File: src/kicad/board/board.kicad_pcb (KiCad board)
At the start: 2 copper layers, 109.4 x 83.4 mm, 50 parts, among them J1 Screw_Terminal_Speaker, J2 Micro_SD_Card_Det, Q1 DMG2301L, SW1 SW_Keyboard, SW2 SW_Keyboard, SW3 RotEncoder_S, SW4 SW_Keyboard, SW5 SW_Keyboard, SW6 Enable BAT, U1 Pico, U2 MAX98357, U3 BQ25172, U5 74HC4051, U6 4072

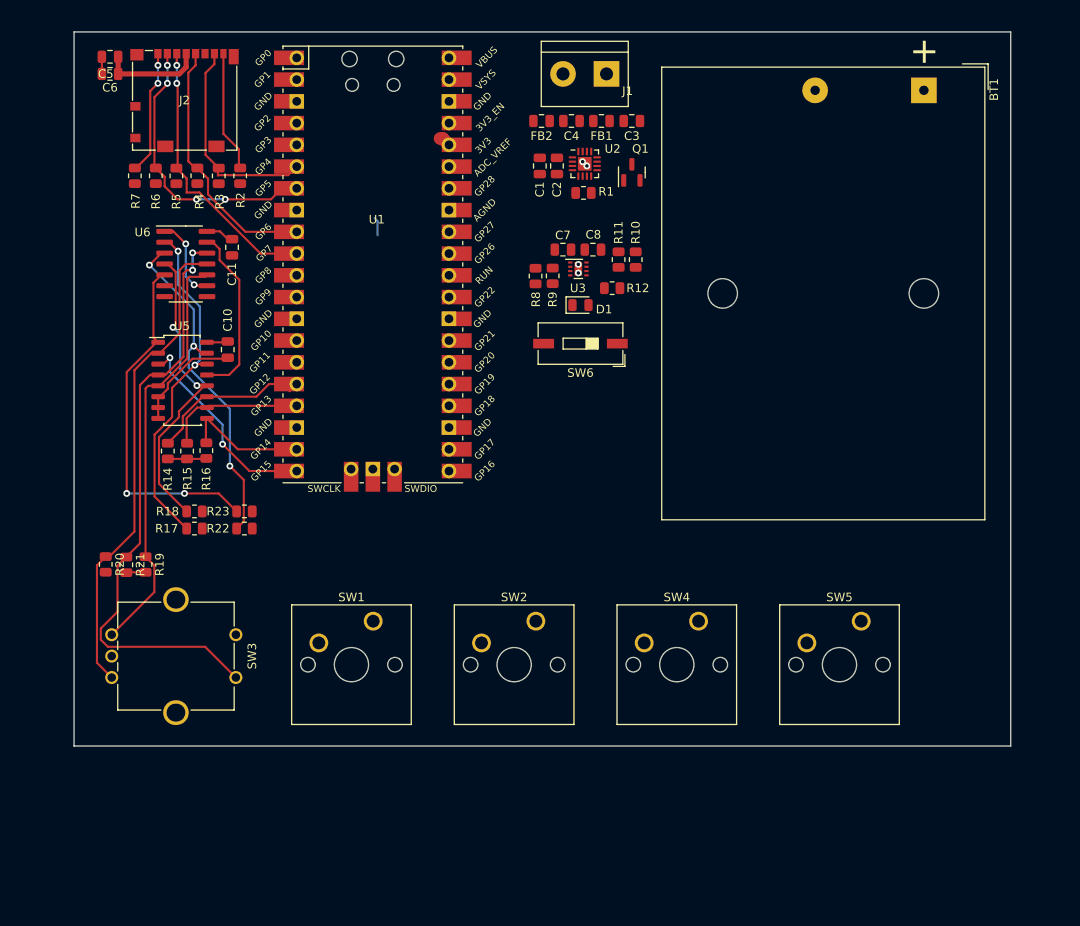
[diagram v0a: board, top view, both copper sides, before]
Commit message: update wip
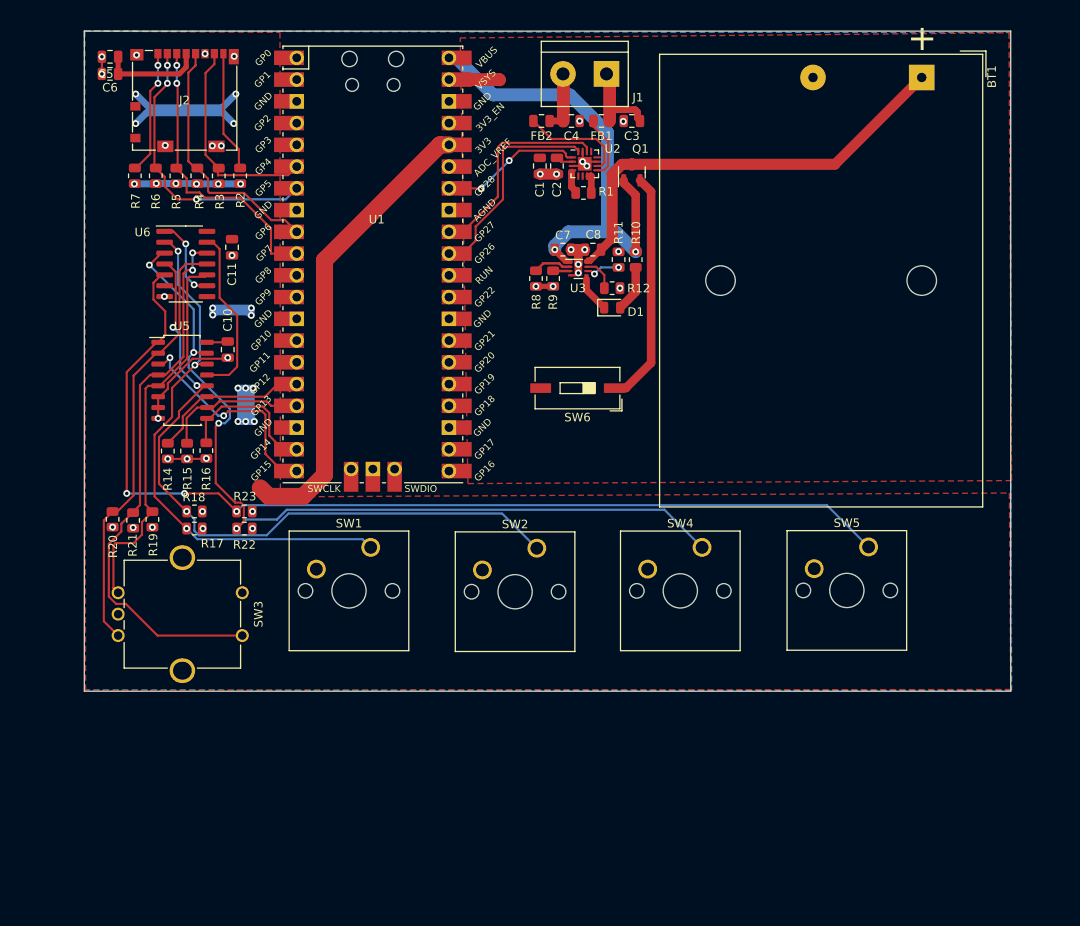
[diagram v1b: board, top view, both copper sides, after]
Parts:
- moved SW5 8.71 mm to (193.4, 97.8)
- moved SW4 8.63 mm to (173.9, 97.8)
- moved SW1 8.62 mm to (135.2, 97.8)
- moved SW2 8.52 mm to (154.7, 97.9)
- moved R19 5.32 mm to (109.8, 94.5)
- moved R20 5.32 mm to (105.1, 94.5)
- moved R21 5.25 mm to (107.5, 94.7)
- moved SW6 5.21 mm to (159.4, 79.2)
- moved SW3 4.96 mm to (105.8, 103.1)
- moved D1 3.71 mm to (163.4, 69.8)
- moved BT1 1.52 mm to (199.6, 42.9)
- moved R9 0.32 mm to (156.6, 66.4)
- moved R8 0.29 mm to (154.6, 66.4)
- turned R10 to -90 degrees
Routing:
- net +3.3V: track 19.0 -> 135.6 mm, vias 0 -> 20
- net B3: track 41.9 -> 118.7 mm, vias 2 -> 3
- net /Power2/USB_VBUS: track 0.00 -> 64.4 mm, vias 0 -> 2
- net B1: track 40.4 -> 99.7 mm, vias 3 -> 4
- net Net-(BT1-Pad1): track 0.00 -> 55.9 mm
- net B2: track 35.9 -> 81.5 mm, vias 2 -> 3
- net Net-(Q1-Pad2): track 0.00 -> 27.4 mm
- net GP26: track 0.00 -> 25.1 mm
- net GP27: track 0.00 -> 24.5 mm
- net B0: track 40.7 -> 63.4 mm, vias 2 -> 3
- net GP28: track 0.00 -> 16.8 mm, vias 0 -> 2
- net Net-(FB2-Pad1): track 0.00 -> 12.4 mm
- net Net-(C3-Pad1): track 0.00 -> 11.2 mm
- net GND: track 21.7 -> 32.3 mm, vias 4 -> 36
- net VDD: track 0.00 -> 10.3 mm
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- added copper zone on F.Cu, net +3.3V
- added copper zone on B.Cu, net GND
- added copper zone on F.Cu, net VDD
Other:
- board size 109.4 x 83.4 mm -> 108.2 x 77.1 mm

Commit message: update
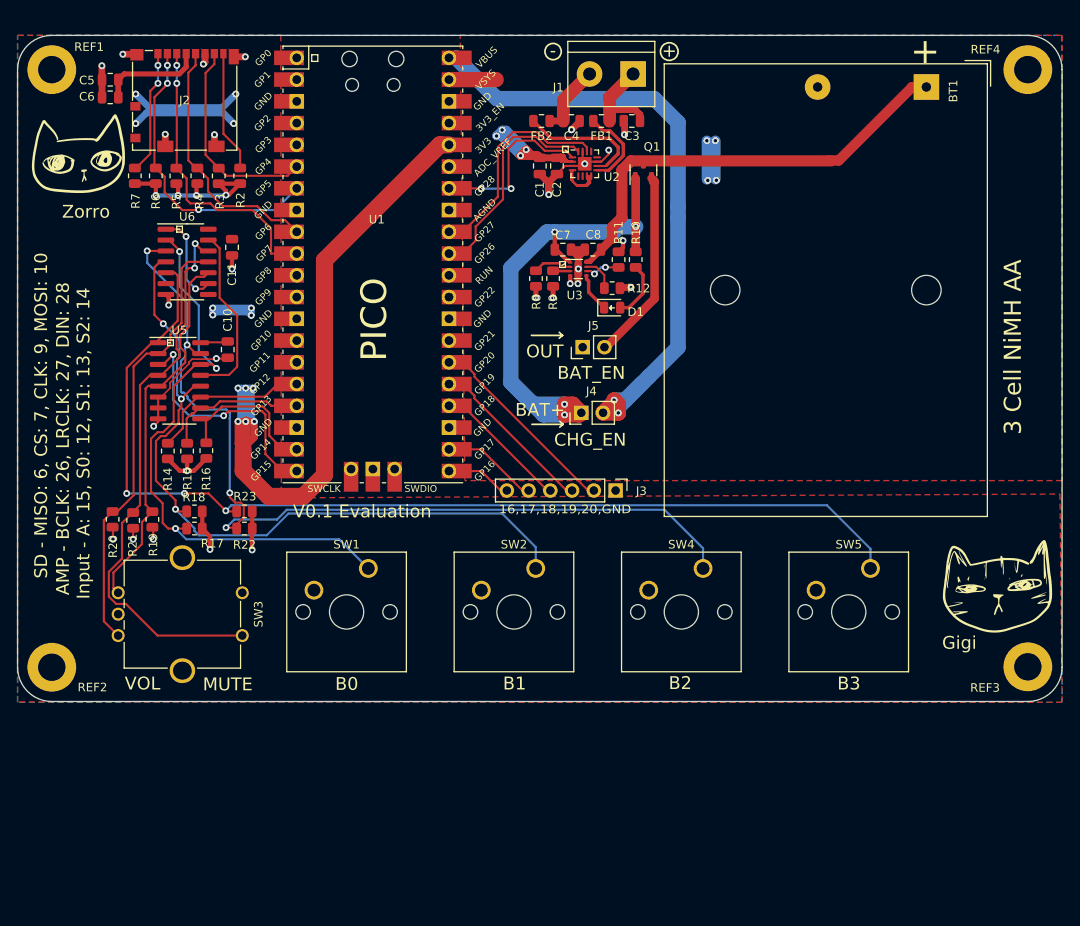
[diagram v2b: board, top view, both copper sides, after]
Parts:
- removed R1: 1M, Resistor_SMD:R_0805_2012Metric
- removed SW6: Enable BAT, Button_Switch_SMD:SW_DIP_SPSTx01_Slide_9.78x4.72mm_W8.61mm_P2.54mm
- added J3: Conn_01x06, Connector_PinHeader_2.54mm:PinHeader_1x06_P2.54mm_Vertical, F.Cu at (163.8, 91.2)
- added J4: Conn_01x02_Male, Connector_PinHeader_2.54mm:PinHeader_1x02_P2.54mm_Vertical, F.Cu at (159.8, 82.1)
- added J5: Conn_01x02_Male, Connector_PinHeader_2.54mm:PinHeader_1x02_P2.54mm_Vertical, F.Cu at (160.0, 74.4)
- added REF1: MountingHole_3.2mm_M3_ISO7380_Pad, MountingHole:MountingHole_3.2mm_M3_ISO7380_Pad, F.Cu at (98.0, 42.0)
- added REF2: MountingHole_3.2mm_M3_ISO7380_Pad, MountingHole:MountingHole_3.2mm_M3_ISO7380_Pad, F.Cu at (98.0, 111.8)
- added REF3: MountingHole_3.2mm_M3_ISO7380_Pad, MountingHole:MountingHole_3.2mm_M3_ISO7380_Pad, F.Cu at (212.0, 111.8)
- added REF4: MountingHole_3.2mm_M3_ISO7380_Pad, MountingHole:MountingHole_3.2mm_M3_ISO7380_Pad, F.Cu at (212.0, 42.0)
- Q1: value DMG2301L -> DMG2305UX
- R10: value 10K -> 1K
- R11: value 8.2K -> 20K
- R12: value 36K -> 20K
- U2: footprint Library:MAX98357 -> Package_DFN_QFN:TQFN-16-1EP_3x3mm_P0.5mm_EP1.6x1.6mm
- U3: footprint Library:BQ25172 -> Package_SON:WSON-8-1EP_2x2mm_P0.5mm_EP0.9x1.6mm
- U5: footprint Library:74HC4051 -> Package_SO:SOIC-16_3.9x9.9mm_P1.27mm
- U6: footprint Library:CD4072BM96 -> Package_SO:SOIC-14_3.9x8.7mm_P1.27mm
- moved J1 3.10 mm to (165.9, 42.5)
- moved C6 2.74 mm to (104.8, 45.2)
- moved C5 2.68 mm to (104.8, 43.2)
- moved SW5 2.52 mm to (193.6, 100.3)
- moved SW1 2.48 mm to (135.0, 100.3)
- moved SW4 2.46 mm to (174.1, 100.3)
- moved SW2 2.36 mm to (154.5, 100.3)
- moved Q1 1.37 mm to (167.1, 53.8)
- moved BT1 1.24 mm to (200.2, 44.0)
- moved U5 0.33 mm to (112.9, 78.3)
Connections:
- C7 pad 1: /Power2/USB_VBUS -> Net-(C7-Pad1)
- Q1 pad 1: /Power2/USB_VBUS -> Net-(C7-Pad1)
- R10 pad 1: /Power2/USB_VBUS -> Net-(C7-Pad1)
- U1 pad 13: unconnected-(U1-Pad13) -> GND
- U1 pad 18: unconnected-(U1-Pad18) -> GND
- U1 pad 21: unconnected-(U1-Pad21) -> Net-(J3-Pad6)
- U1 pad 22: unconnected-(U1-Pad22) -> Net-(J3-Pad5)
- U1 pad 23: unconnected-(U1-Pad23) -> GND
- U1 pad 24: unconnected-(U1-Pad24) -> Net-(J3-Pad4)
- U1 pad 25: unconnected-(U1-Pad25) -> Net-(J3-Pad3)
- U1 pad 26: unconnected-(U1-Pad26) -> Net-(J3-Pad2)
- U1 pad 28: unconnected-(U1-Pad28) -> GND
- U1 pad 3: unconnected-(U1-Pad3) -> GND
- U1 pad 33: unconnected-(U1-Pad33) -> GND
- U1 pad 38: unconnected-(U1-Pad38) -> GND
- U1 pad 8: unconnected-(U1-Pad8) -> GND
- U2 pad 4: Net-(R1-Pad2) -> VDD
- U3 pad 1: /Power2/USB_VBUS -> Net-(C7-Pad1)
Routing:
- net Net-(C7-Pad1): track 0.00 -> 65.8 mm, vias 0 -> 4
- net GND: track 32.3 -> 80.5 mm, vias 36 -> 28
- net VDD: track 10.3 -> 51.5 mm, vias 0 -> 8
- net +3.3V: track 135.6 -> 162.3 mm, vias 20 -> 18
- net Net-(J3-Pad2): track 0.00 -> 22.6 mm
- net Net-(J3-Pad3): track 0.00 -> 19.0 mm
- net Net-(J3-Pad4): track 0.00 -> 15.4 mm
- net /Power2/USB_VBUS: track 64.4 -> 79.5 mm
- net Net-(J3-Pad5): track 0.00 -> 10.5 mm
- net Net-(J3-Pad6): track 0.00 -> 6.93 mm
- net B0: track 63.4 -> 70.2 mm
- net B1: track 99.7 -> 105.8 mm
- net Net-(Q1-Pad2): track 27.4 -> 22.0 mm
- net B2: track 81.5 -> 86.8 mm
- net B3: track 118.7 -> 123.5 mm
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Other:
- board size 108.2 x 77.1 mm -> 122 x 77.8 mm
- board text added: "+"
- board text added: "-"
- board text added: "16,17,18,19,20,GND"
- board text added: "3 Cell NiMH AA"
- board text added: "AMP - BCLK: 26, LRCLK: 27, DIN: 28"
- board text added: "B0"
- board text added: "B1"
- board text added: "B2"
- board text added: "B3"
- board text added: "BAT+"
- board text added: "BAT_EN"
- board text added: "CHG_EN"
- board text added: "Gigi"
- board text added: "Input - A: 15, S0: 12, S1: 13, S2: 14"
- board text added: "MUTE"
- board text added: "OUT"
- board text added: "PICO"
- board text added: "SD - MISO: 6, CS: 7, CLK: 9, MOSI: 10"
- board text added: "V0.1 Evaluation"
- board text added: "VOL"
- board text added: "Zorro"

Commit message: update
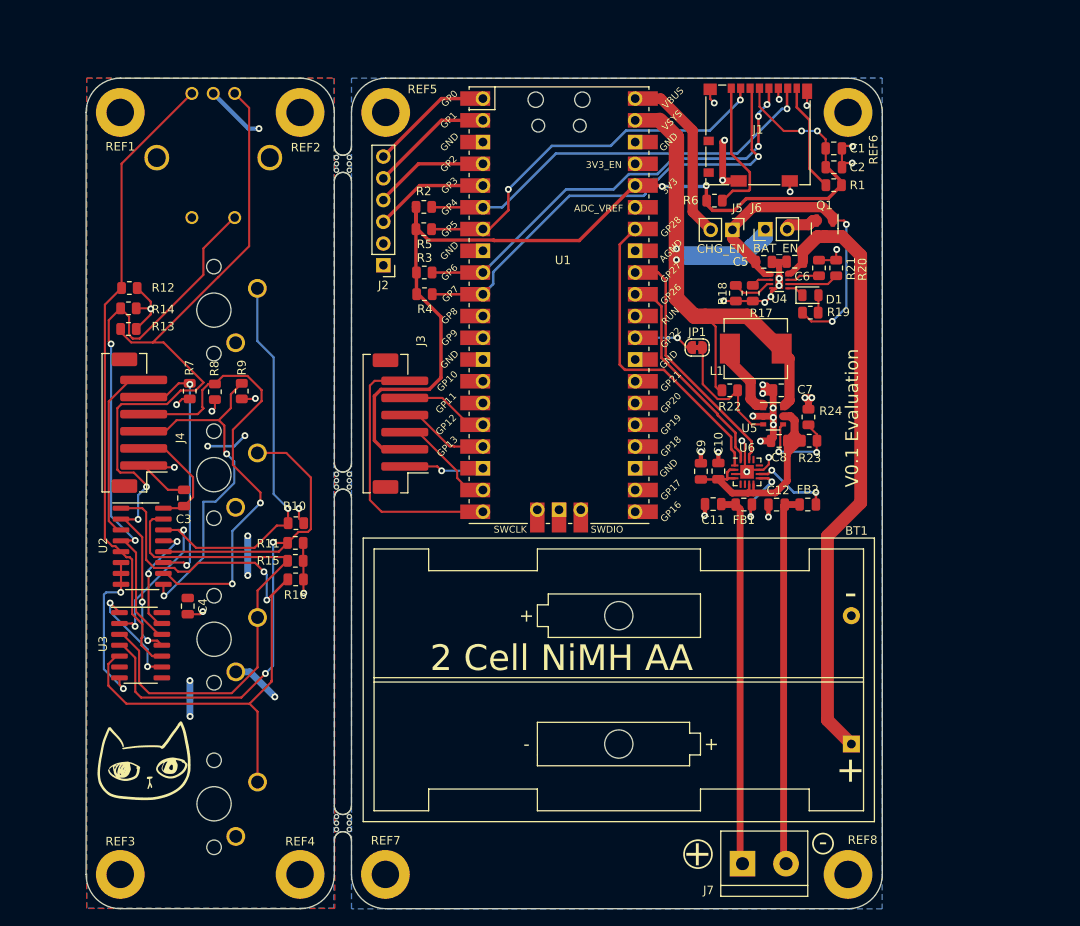
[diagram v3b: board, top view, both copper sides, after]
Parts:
- added C12: 220pF, Capacitor_SMD:C_0805_2012Metric, F.Cu at (182.7, 92.8)
- added C9: 10uF, Capacitor_SMD:C_0805_2012Metric, F.Cu at (173.8, 88.9)
- added J6: Conn_01x02_Male, Connector_PinHeader_2.54mm:PinHeader_1x02_P2.54mm_Vertical, F.Cu at (181.3, 60.6)
- added J7: Screw_Terminal_Speaker, TerminalBlock:TerminalBlock_bornier-2_P5.08mm, F.Cu at (178.7, 134.7)
- added JP1: Boost EN Connect, Jumper:SolderJumper-2_P1.3mm_Bridged_RoundedPad1.0x1.5mm, F.Cu at (173.4, 74.5)
- added L1: 2.2uH, Inductor_SMD:L_Sunlord_MWSA06xxS, F.Cu at (180.2, 74.6)
- added R1: 47K, Resistor_SMD:R_0805_2012Metric, F.Cu at (189.3, 55.5)
- added R13: 10K, Resistor_SMD:R_0805_2012Metric, F.Cu at (107.0, 72.3)
- added R24: 10K, Resistor_SMD:R_0805_2012Metric, F.Cu at (186.4, 82.6)
- added REF5: MountingHole_3.2mm_M3_ISO7380_Pad, MountingHole:MountingHole_3.2mm_M3_ISO7380_Pad, F.Cu at (137.0, 47.0)
- added REF6: MountingHole_3.2mm_M3_ISO7380_Pad, MountingHole:MountingHole_3.2mm_M3_ISO7380_Pad, F.Cu at (191.0, 47.0)
- added REF7: MountingHole_3.2mm_M3_ISO7380_Pad, MountingHole:MountingHole_3.2mm_M3_ISO7380_Pad, F.Cu at (137.0, 136.0)
- added REF8: MountingHole_3.2mm_M3_ISO7380_Pad, MountingHole:MountingHole_3.2mm_M3_ISO7380_Pad, F.Cu at (191.0, 136.0)
- added U4: BQ25172, Package_SON:WSON-8-1EP_2x2mm_P0.5mm_EP0.9x1.6mm, F.Cu at (183.0, 66.8)
- added mouse-bite-2mm-slot: VAL1, Library:mouse-bite-2mm-slot, F.Cu at (132.0, 90.0)
- added mouse-bite-2mm-slot: VAL2, Library:mouse-bite-2mm-slot, F.Cu at (132.0, 53.0)
- added mouse-bite-2mm-slot: VAL3, Library:mouse-bite-2mm-slot, F.Cu at (132.0, 130.0)
- BT1: footprint Battery:BatteryHolder_Keystone_2479_3xAAA -> Battery:BatteryHolder_Keystone_2462_2xAA
- C11: value 0.1uF -> 220pF
- C3, C4: value 220pF -> 0.1uF
- C6: value 0.1uF -> 10uF
- C8: value 10uF -> 22uF
- J1: value Screw_Terminal_Speaker -> Micro_SD_Card_Det; footprint TerminalBlock:TerminalBlock_bornier-2_P5.08mm -> Connector_Card:microSD_HC_Molex_104031-0811
- J2: value Micro_SD_Card_Det -> Conn_01x06; footprint Connector_Card:microSD_HC_Molex_104031-0811 -> Connector_PinHeader_2.54mm:PinHeader_1x06_P2.54mm_Vertical
- J3: value Conn_01x06 -> Conn_01x06_Male; footprint Connector_PinHeader_2.54mm:PinHeader_1x06_P2.54mm_Vertical -> Connector_JST:JST_PH_B6B-PH-SM4-TB_1x06-1MP_P2.00mm_Vertical
- J4: value Conn_01x02_Male -> Conn_01x06_Male; footprint Connector_PinHeader_2.54mm:PinHeader_1x02_P2.54mm_Vertical -> Connector_JST:JST_PH_B6B-PH-SM4-TB_1x06-1MP_P2.00mm_Vertical
- R10: value 1K -> 10K
- R11, R12: value 20K -> 10K
- R14, R15, R16: value 2K7 -> 10K
- R17, R19: value 10K -> 1K
- R20, R21: value 10K -> 20K
- R23: value 10K -> 90.9K
- R7: value 47K -> 2K7
- R8: value 1K -> 2K7
- R9: value 10K -> 2K7
- SW1, SW2, SW3, SW4, SW5: moved to B.Cu
- U2: value MAX98357 -> 74HC4051; footprint Package_DFN_QFN:TQFN-16-1EP_3x3mm_P0.5mm_EP1.6x1.6mm -> Package_SO:SOIC-16_3.9x9.9mm_P1.27mm
- U3: value BQ25172 -> 4072; footprint Package_SON:WSON-8-1EP_2x2mm_P0.5mm_EP0.9x1.6mm -> Package_SO:SOIC-14_3.9x8.7mm_P1.27mm
- U5: value 74HC4051 -> TLV61070A; footprint Package_SO:SOIC-16_3.9x9.9mm_P1.27mm -> Package_SO:TSOP-6_1.65x3.05mm_P0.95mm
- U6: value 4072 -> MAX98357; footprint Package_SO:SOIC-14_3.9x8.7mm_P1.27mm -> Package_DFN_QFN:TQFN-16-1EP_3x3mm_P0.5mm_EP1.6x1.6mm
- moved REF4 126.7 mm to (127.0, 136.0)
- moved REF3 108.7 mm to (106.0, 136.0)
- moved R20 89.5 mm to (189.6, 65.2), turned to 90 degrees
- moved R21 85.4 mm to (187.6, 65.2), turned to 90 degrees
- moved C6 82.2 mm to (184.8, 64.4)
- moved R19 80.6 mm to (186.6, 70.4), turned to 0 degrees
- moved C5 79.2 mm to (181.2, 64.5), turned to 0 degrees
- moved BT1 77.2 mm to (191.4, 120.8), turned to 180 degrees
- moved SW5 75.8 mm to (122.0, 125.2), turned to 90 degrees
- moved C4 72.2 mm to (113.9, 104.7), turned to -90 degrees
- moved REF2 71.0 mm to (127.0, 47.0)
- moved R17 70.8 mm to (179.9, 68.1), turned to 90 degrees
- moved U6 69.9 mm to (179.2, 89.0)
- moved U5 69.5 mm to (182.3, 82.5)
- moved C3 68.4 mm to (113.5, 92.0), turned to 90 degrees
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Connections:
- C1 pad 1: VDD -> +3.3V
- C10 pad 1: +3.3V -> VDD
- C11 pad 1: +3.3V -> Net-(C11-Pad1)
- C2 pad 1: VDD -> +3.3V
- C3 pad 1: Net-(C3-Pad1) -> /Input/3.3V_LOCAL
- C3 pad 2: GND -> /Input/GND_LOCAL
- C4 pad 1: GND -> /Input/3.3V_LOCAL
- C4 pad 2: Net-(C4-Pad2) -> /Input/GND_LOCAL
- C5 pad 1: +3.3V -> Net-(C5-Pad1)
- C6 pad 1: +3.3V -> Net-(BT1-Pad1)
- C7 pad 1: Net-(C7-Pad1) -> /Power/OUT
- C8 pad 1: Net-(BT1-Pad1) -> VDD
- FB1 pad 2: Net-(C3-Pad1) -> Net-(C11-Pad1)
- FB2 pad 2: Net-(C4-Pad2) -> Net-(C12-Pad2)
- J1 pad 1: Net-(C3-Pad1) -> Net-(J1-Pad1)
- J1 pad 2: Net-(C4-Pad2) -> SD_CS
- J2 pad 1: Net-(J2-Pad1) -> GND
- J2 pad 2: SD_CS -> GND
- J2 pad 3: SD_MOSI -> Net-(J2-Pad3)
- J2 pad 4: +3.3V -> Net-(J2-Pad4)
- J2 pad 5: SD_CLK -> Net-(J2-Pad5)
- J2 pad 6: GND -> Net-(J2-Pad6)
- J3 pad 2: Net-(J3-Pad2) -> +3.3V
- J3 pad 3: Net-(J3-Pad3) -> GP14
- J3 pad 4: Net-(J3-Pad4) -> GP13
- J3 pad 5: Net-(J3-Pad5) -> GP12
- J3 pad 6: Net-(J3-Pad6) -> GP15
- J4 pad 1: Net-(C7-Pad1) -> /Input/GND_LOCAL
- J4 pad 2: /Power2/USB_VBUS -> /Input/3.3V_LOCAL
- J5 pad 1: VDD -> Net-(C5-Pad1)
- J5 pad 2: Net-(Q1-Pad2) -> /Power/USB_VBUS
- Q1 pad 1: Net-(C7-Pad1) -> Net-(C5-Pad1)
- Q1 pad 2: Net-(Q1-Pad2) -> Net-(J6-Pad2)
- R10 pad 1: Net-(C7-Pad1) -> B0
- R10 pad 2: Net-(D1-Pad2) -> /Input/GND_LOCAL
- R11 pad 1: Net-(R11-Pad1) -> B2
- R11 pad 2: GND -> /Input/GND_LOCAL
- R12 pad 1: Net-(R12-Pad1) -> B4
- R12 pad 2: GND -> /Input/GND_LOCAL
- R14 pad 1: GP12 -> B6
- R14 pad 2: GND -> /Input/GND_LOCAL
- R15 pad 1: GP13 -> B1
- R15 pad 2: GND -> /Input/GND_LOCAL
- R16 pad 1: GP14 -> B3
- R16 pad 2: GND -> /Input/GND_LOCAL
- R17 pad 1: B0 -> GND
- R17 pad 2: GND -> Net-(R17-Pad2)
- R18 pad 1: B2 -> GND
- R18 pad 2: GND -> Net-(R18-Pad2)
- R19 pad 1: B4 -> Net-(C5-Pad1)
- R19 pad 2: GND -> Net-(D1-Pad2)
- R2 pad 2: Net-(J2-Pad8) -> SD_MISO
- R20 pad 1: B5 -> Net-(R20-Pad1)
- R21 pad 1: B6 -> Net-(R21-Pad1)
- R22 pad 1: B1 -> /Power/OUT
- R22 pad 2: GND -> Net-(JP1-Pad2)
- R23 pad 1: B3 -> VDD
- R23 pad 2: GND -> Net-(R23-Pad2)
- R3 pad 2: SD_MISO -> SD_CLK
- R4 pad 2: SD_CLK -> SD_MOSI
- R5 pad 2: SD_MOSI -> SD_CS
- R6 pad 2: SD_CS -> Net-(J1-Pad1)
- R7 pad 1: +3.3V -> /Input/S0
- R7 pad 2: Net-(J2-Pad1) -> /Input/GND_LOCAL
- R8 pad 1: GND -> /Input/S1
- R8 pad 2: Net-(R8-Pad2) -> /Input/GND_LOCAL
- R9 pad 1: GND -> /Input/S2
- R9 pad 2: Net-(R9-Pad2) -> /Input/GND_LOCAL
- SW1 pad 2: +3.3V -> /Input/3.3V_LOCAL
- SW2 pad 2: +3.3V -> /Input/3.3V_LOCAL
- SW3 pad C: +3.3V -> /Input/3.3V_LOCAL
- SW3 pad S1: +3.3V -> /Input/3.3V_LOCAL
- SW4 pad 2: +3.3V -> /Input/3.3V_LOCAL
- SW5 pad 2: +3.3V -> /Input/3.3V_LOCAL
- U1 pad 1: unconnected-(U1-Pad1) -> Net-(J2-Pad6)
- U1 pad 2: unconnected-(U1-Pad2) -> Net-(J2-Pad5)
- U1 pad 21: Net-(J3-Pad6) -> unconnected-(U1-Pad21)
- U1 pad 22: Net-(J3-Pad5) -> unconnected-(U1-Pad22)
- U1 pad 24: Net-(J3-Pad4) -> unconnected-(U1-Pad24)
- U1 pad 25: Net-(J3-Pad3) -> unconnected-(U1-Pad25)
- U1 pad 26: Net-(J3-Pad2) -> unconnected-(U1-Pad26)
- U1 pad 29: unconnected-(U1-Pad29) -> /Sound/SPEAKER_EN
- U1 pad 39: VDD -> /Power/OUT
- U1 pad 4: unconnected-(U1-Pad4) -> Net-(J2-Pad4)
- U1 pad 40: /Power2/USB_VBUS -> /Power/USB_VBUS
- U1 pad 5: unconnected-(U1-Pad5) -> Net-(J2-Pad3)
- U2 pad 1: GP28 -> B3
- U2 pad 10: Net-(FB2-Pad1) -> /Input/S1
- U2 pad 11: GND -> /Input/S0
- U2 pad 12: (no net) -> B2
- U2 pad 13: (no net) -> ANY
- U2 pad 14: GP27 -> B0
- U2 pad 15: GND -> B1
- U2 pad 16: GP26 -> /Input/3.3V_LOCAL
- U2 pad 2: VDD -> B5
- U2 pad 3: GND -> /Input/A
- U2 pad 4: VDD -> B6
- U2 pad 5: (no net) -> B4
- U2 pad 6: (no net) -> /Input/GND_LOCAL
- U2 pad 7: VDD -> /Input/GND_LOCAL
- U2 pad 8: VDD -> /Input/GND_LOCAL
- U2 pad 9: Net-(FB1-Pad1) -> /Input/S2
- U3 pad 1: Net-(C7-Pad1) -> Net-(U3-Pad1)
- U3 pad 2: Net-(R8-Pad2) -> B0
- U3 pad 3: Net-(R9-Pad2) -> B1
- U3 pad 4: GND -> B2
- U3 pad 5: Net-(D1-Pad1) -> B3
- U3 pad 6: Net-(R11-Pad1) -> (no net)
- U3 pad 7: Net-(R12-Pad1) -> /Input/GND_LOCAL
- U3 pad 8: Net-(BT1-Pad1) -> (no net)
- U3 pad 9: GND -> Net-(U3-Pad1)
- U5 pad 1: B3 -> Net-(L1-Pad2)
- U5 pad 2: B5 -> GND
- U5 pad 3: GP15 -> Net-(JP1-Pad2)
- U5 pad 4: B6 -> Net-(R23-Pad2)
- U5 pad 5: B4 -> VDD
- U5 pad 6: GND -> /Power/OUT
- U6 pad 1: Net-(U6-Pad1) -> GP28
- U6 pad 10: B4 -> Net-(FB2-Pad1)
- U6 pad 11: B5 -> GND
- U6 pad 12: B6 -> (no net)
- U6 pad 13: ANY -> (no net)
- U6 pad 14: +3.3V -> GP27
- U6 pad 2: B0 -> VDD
- U6 pad 3: B1 -> GND
- U6 pad 4: B2 -> VDD
- U6 pad 5: B3 -> (no net)
- U6 pad 7: GND -> VDD
- U6 pad 8: (no net) -> VDD
- U6 pad 9: Net-(U6-Pad1) -> Net-(FB1-Pad1)
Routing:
- net /Power/OUT: track 0.00 -> 82.3 mm, vias 0 -> 2
- net /Power2/USB_VBUS: track 79.5 -> 0.00 mm, vias 2 -> 0
- net Net-(C7-Pad1): track 65.8 -> 0.00 mm, vias 4 -> 0
- net /Input/S1: track 0.00 -> 53.0 mm, vias 0 -> 2
- net /Input/GND_LOCAL: track 0.00 -> 51.1 mm, vias 0 -> 10
- net B1: track 105.8 -> 58.2 mm, vias 4 -> 0
- net B3: track 123.5 -> 78.3 mm, vias 3 -> 2
- net +3.3V: track 162.3 -> 117.8 mm, vias 18 -> 4
- net Net-(C11-Pad1): track 0.00 -> 43.4 mm
- net Net-(C12-Pad2): track 0.00 -> 43.2 mm
- net /Input/S2: track 0.00 -> 41.7 mm, vias 0 -> 2
- net B5: track 52.1 -> 93.6 mm, vias 0 -> 4
- net /Input/3.3V_LOCAL: track 0.00 -> 40.1 mm, vias 0 -> 8
- net Net-(C5-Pad1): track 0.00 -> 39.1 mm, vias 0 -> 2
- net /Input/S0: track 0.00 -> 30.2 mm, vias 0 -> 2
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- added copper zone on F.Cu, net /Input/3.3V_LOCAL
- added copper zone on B.Cu, net /Input/GND_LOCAL
- removed copper zone on F.Cu, net +3.3V
- removed copper zone on F.Cu, net VDD
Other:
- board size 122 x 77.8 mm -> 93 x 97 mm
- board text added: "2 Cell NiMH AA"
- board text added: "PLACE OTHER SIDE"
- board text removed: "16,17,18,19,20,GND"
- board text removed: "3 Cell NiMH AA"
- board text removed: "Gigi"
- board text removed: "OUT"
- board text removed: "PICO"
- board text removed: "Zorro"
